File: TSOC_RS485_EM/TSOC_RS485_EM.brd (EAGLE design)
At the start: 43.2 x 25.4 mm, 54 parts, among them Q1 FDC6420C, Q2 MOSFET-NCHANNELAO3404A, U1 ST1480ACSOIC, U2 ATMEGA328, U3 MIC5219 3.3V, U4 NCP361SNT1G, X1 8MHZ

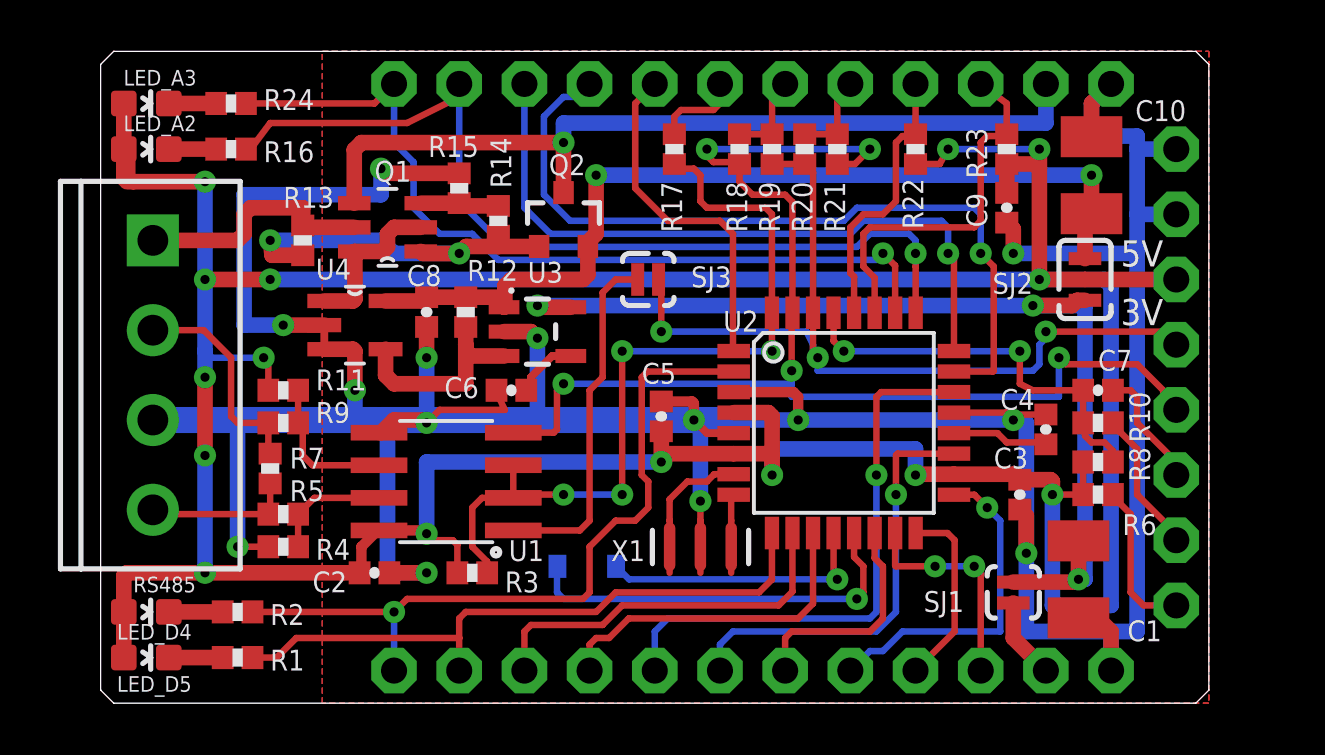
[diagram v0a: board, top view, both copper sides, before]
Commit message: update to revision 5.0
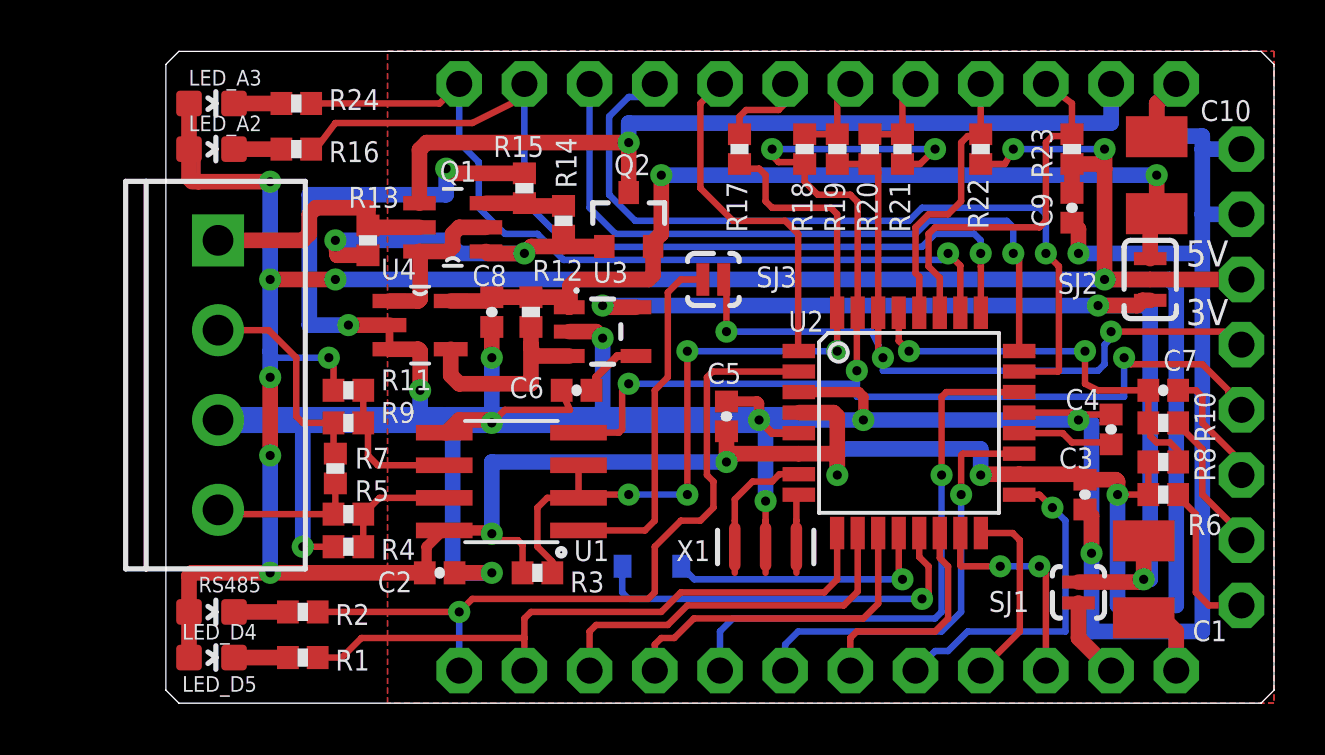
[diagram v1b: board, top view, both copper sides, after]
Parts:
- moved C5 2.54 mm to (21.8, 11.2)
- moved R21 2.54 mm to (28.7, 21.6)
- moved D9 2.54 mm to (17.8, 5.33)
- moved Q1 2.54 mm to (11.2, 18.5)
- moved R12 2.54 mm to (14.2, 15.2)
- moved R15 2.54 mm to (14.0, 20.1)
- moved U3 2.54 mm to (17.0, 14.5)
- moved U4 2.54 mm to (9.91, 14.7)
- moved LED_A2 2.54 mm to (1.78, 21.6)
- moved LED_A3 2.54 mm to (1.78, 23.4)
- moved LED_D4 2.54 mm to (1.78, 3.56)
- moved LED_D5 2.54 mm to (1.78, 1.78)
- moved R11 2.54 mm to (7.11, 12.2)
- moved R13 2.54 mm to (7.87, 18.0)
- moved R16 2.54 mm to (5.08, 21.6)
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
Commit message: update to Rev6.0
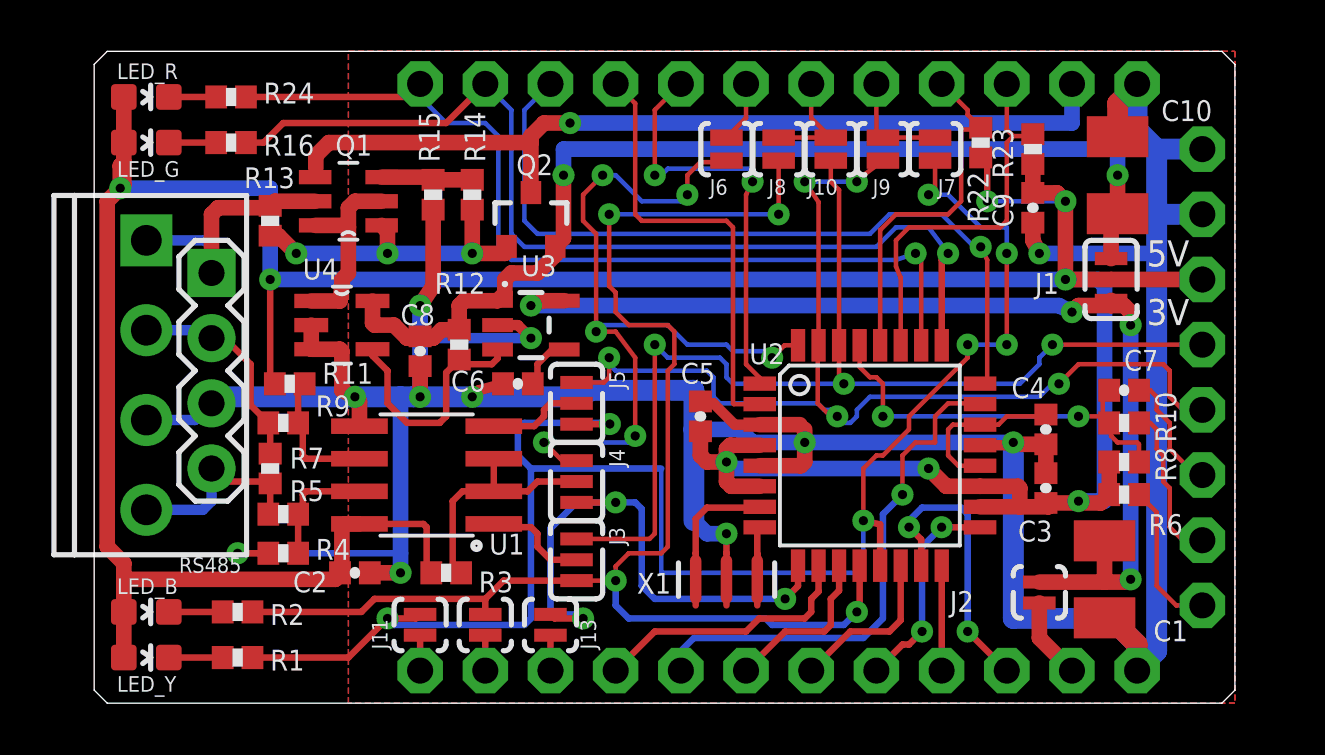
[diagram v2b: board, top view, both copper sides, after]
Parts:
- removed D8, D9: (no value), PatternAgents-ProtoPads:WPAD-1-0402
- removed LED_A2, LED_A3, LED_D4, LED_D5: (no value), TSOC-MODBUS-ESM:LED-0603
- removed R17, R18, R19, R20, R21: DNP, TSOC-MODBUS-ESM:0402-RES
- removed SJ1, SJ3: JMP-2-NC, TSOC-MODBUS-ESM:JMP-2-NC
- removed SJ2: JMP-3-1_2, PatternAgents-ProtoPads:JMP-3-1_2
- added J1: JMP-3-1_2, PatternAgents-ProtoPads:JMP-3-1_2
- added J10, J6, J7, J8, J9: (no value), TSOC_RS485_EM:JMP-2-NO
- added J11, J12, J13, J2: JMP-2-NC, TSOC-MODBUS-ESM:JMP-2-NC
- added J3, J4, J5: JMP-3-1_2, TSOC_RS485_EM:JMP-3-1_2
- added JP1: (no value), TSOC_RS485_EM:1X04
- added LED_B, LED_G, LED_R, LED_Y: (no value), TSOC-MODBUS-ESM:LED-0603
- RS485: device SparkFun-Connectors:SCREWTERMINAL-3.5MM-4 -> TSOC_RS485_EM:SCREWTERMINAL-3.5MM-4
- U$1: value TSOC-PCB-EM-BB -> TSOC-PCB-EM-45; device TSOC_RS485_EM:TSOC-EM-BB -> TSOC_RS485_EM:TSOC-EM-BB-45MM
- moved Q1 4.19 mm to (7.11, 19.6)
- moved R13 3.89 mm to (4.06, 18.8)
- moved Q2 3.81 mm to (14.2, 18.8)
- moved R14 3.70 mm to (11.9, 19.8)
- moved R15 3.57 mm to (10.4, 19.8), turned to 270 degrees
- moved R3 3.56 mm to (10.9, 5.08)
- moved U1 3.31 mm to (10.2, 8.89)
- moved C2 3.30 mm to (7.37, 5.08)
- moved C8 3.18 mm to (9.91, 13.7)
- moved R12 3.07 mm to (11.4, 14.0)
- moved U4 3.05 mm to (6.86, 14.7)
- moved U3 2.81 mm to (14.2, 14.7)
- moved RS485 2.79 mm to (-0.76, 18.0)
- moved R16 2.55 mm to (2.54, 21.8)
- moved R24 2.55 mm to (2.54, 23.6)
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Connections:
- removed net A6: TSOC.6B, U2.19
- removed net A7: TSOC.5B, U2.22
- new net DE: J4.2, R3.1, U1.2, U1.3
- new net DI: J5.2, U1.4
- new net N$1: J13.1, TSOC.3B
- new net TSOC_D8: J12.1, TSOC.2B
- new net TSOC_D9: J11.1, TSOC.1B
- net 3V3: now also J1.1, J2.1; no longer SJ1.1, SJ2.1
- net 5V0: now also J1.3; no longer SJ2.3
- net A0: now also TSOC.5B; no longer TSOC.4C
- net AO: now also JP1.2
- net AREF: now also U2.22
- net BO: now also JP1.4
- net D0: now also J10.2, J3.1; no longer R19.2, R20.2, SJ3.1
- net D1: now also J5.1, J9.2; no longer R18.2, R21.2, U1.4
- net D2: now also J4.1, J6.2; no longer R17.2, R3.1, U1.2, U1.3
- net D4: now also TSOC.4C; no longer R2.2, TSOC.1B
- net D5: now also J13.2, J4.3; no longer R1.2, TSOC.2B
- net D6: now also TSOC.4B; no longer TSOC.3B
- net D7: now also TSOC.6B; no longer TSOC.4B
- net D8: now also J12.2, J3.3, J8.2, R2.2; no longer D8.1
- net D9: now also J11.2, J5.3, J7.2, R1.2; no longer D9.1
- net EXT_5V0: now also JP1.1
- net GND: now also JP1.3
- net LEDB: now also LED_B.C; no longer LED_D4.C
- net LEDG: now also LED_G.C; no longer LED_A2.C
- net LEDR: now also LED_R.C; no longer LED_A3.C
- net LEDY: now also LED_Y.C; no longer LED_D5.C
- net RXD: now also J3.2; no longer SJ3.2
- net TSOC_3V3: now also J2.2; no longer SJ1.2
- net TSOC_CTS: now also J6.1; no longer R17.1
- net TSOC_RXD: now also J10.1, J8.1; no longer R18.1, R19.1
- net TSOC_TXD: now also J7.1, J9.1; no longer R20.1, R21.1
- net VCC: now also J1.2, LED_B.A, LED_G.A, LED_R.A, LED_Y.A, U2.19; no longer LED_A2.A, LED_A3.A, LED_D4.A, LED_D5.A, SJ2.2
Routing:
- net D9: track 15.6 -> 66.7 mm, vias 1 -> 7
- net D8: track 10.7 -> 54.6 mm, vias 1 -> 4
- net A7: track 22.0 -> 0.00 mm, vias 1 -> 0
- net VCC: track 156.2 -> 136.1 mm, vias 15 -> 8
- net GND: track 159.4 -> 141.4 mm, vias 14 -> 11
- net A6: track 16.8 -> 0.00 mm, vias 1 -> 0
- net D4: track 29.3 -> 17.3 mm, vias 1 -> 0
- net A0: track 31.0 -> 20.3 mm
- net RXD: track 13.8 -> 4.10 mm
- net DE: track 0.00 -> 9.34 mm
- net D0: track 33.8 -> 42.8 mm
- net D1: track 50.7 -> 42.5 mm
- net D7: track 13.1 -> 6.48 mm
- net D13: track 13.0 -> 8.29 mm, vias 1 -> 2
- net 5V0: track 36.3 -> 40.7 mm
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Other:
- board size 43.2 x 25.4 mm -> 44.4 x 25.4 mm
- board text added: "D8"
- board text added: "D9"
- board text added: "MAX 6Vdc"
- board text added: "Rev 6.0 (AVR Version)"
- board text removed: "A6"
- board text removed: "A7"
- board text removed: "Rev 5.0 (AVR Version)"
